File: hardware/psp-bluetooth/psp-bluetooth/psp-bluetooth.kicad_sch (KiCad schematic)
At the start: 16 parts, among them J1 Left Connector, J2 Center Connector, J3 Right Connector, J4 Analog Connector, J5 PSP Power out, J6 Power IN, J7 Serial, J8 Vin Toggle, P1 Digital, P2 Analog, P3 CONN_01X01, P4 CONN_01X01, P5 CONN_01X01, P6 CONN_01X01, U1 MCP4251-xxxx-P

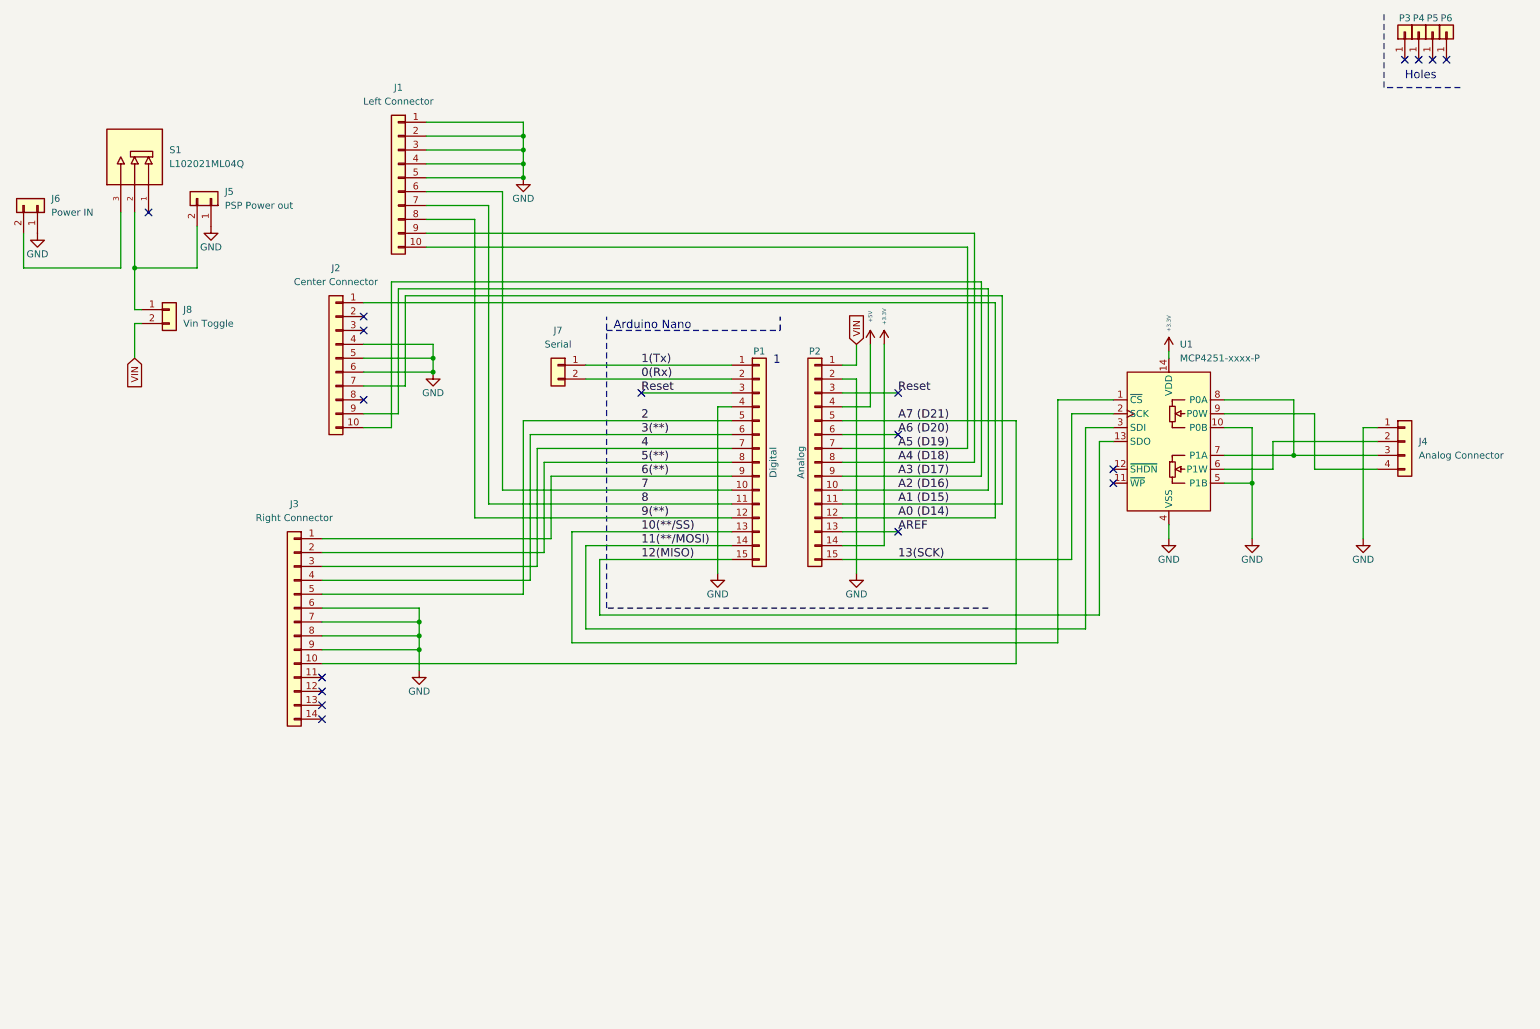
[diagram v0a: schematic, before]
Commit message: Initial work and hardware stuff
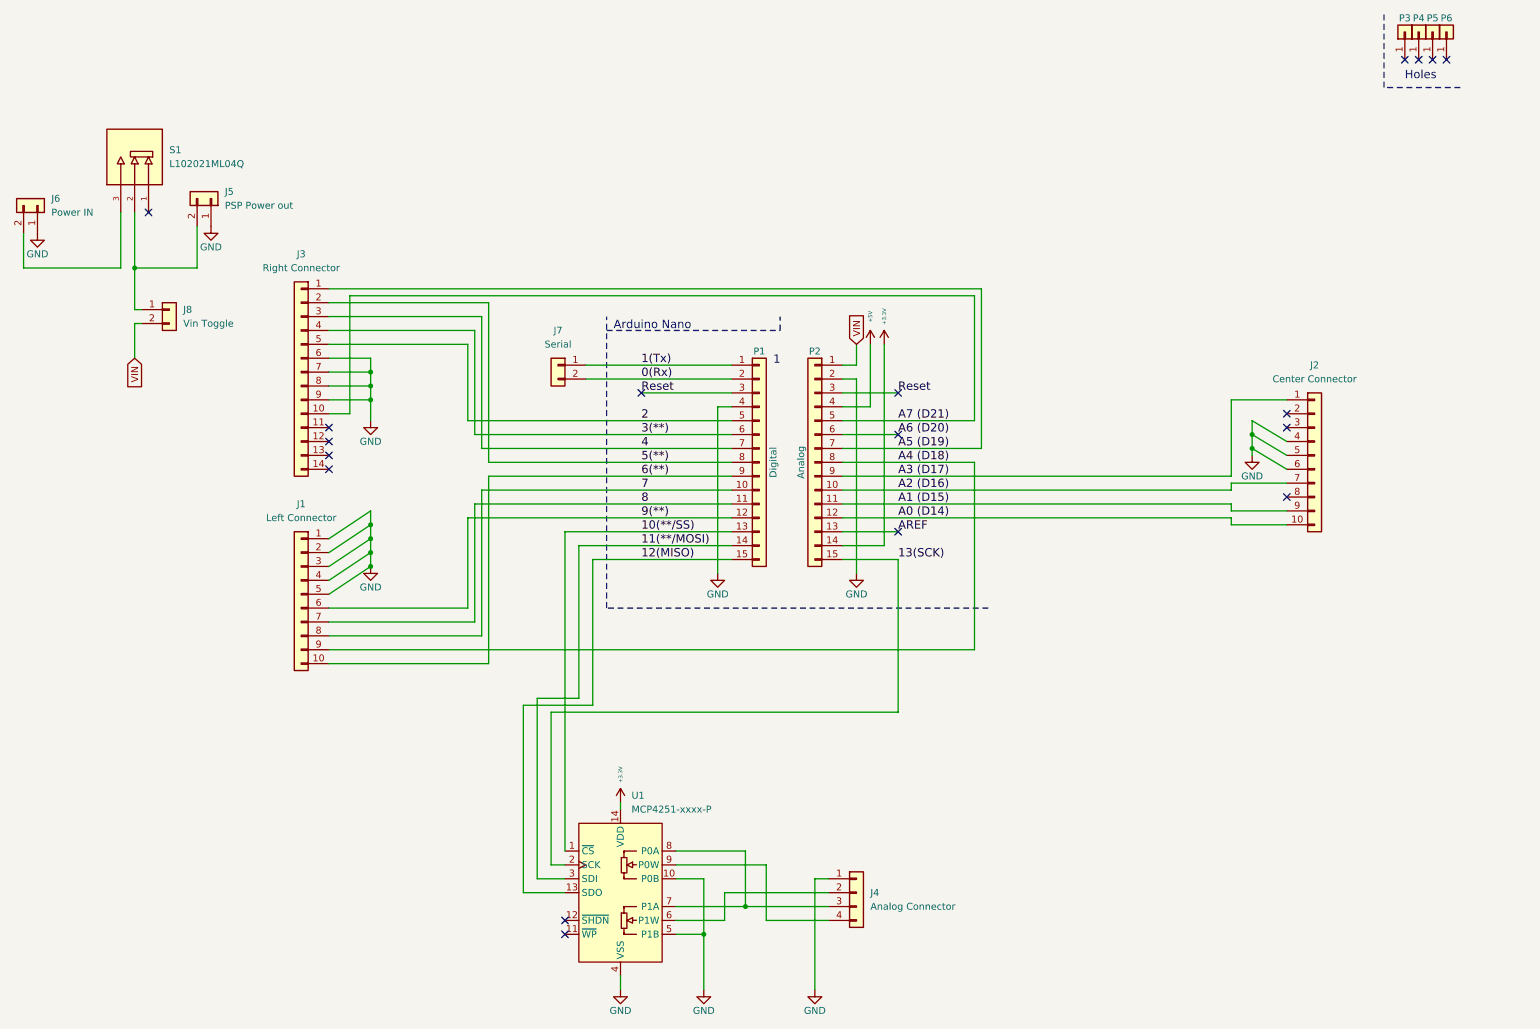
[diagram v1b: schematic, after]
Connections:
- net 6(**): now also J1.10 (Pin_10); no longer J3.1 (Pin_1)
- net 7: now also J1.8 (Pin_8); no longer J1.6 (Pin_6)
- net 9(**): now also J1.6 (Pin_6); no longer J1.8 (Pin_8)
- net A0 (D14): now also J2.10 (Pin_10); no longer J2.1 (Pin_1)
- net A1 (D15): now also J2.9 (Pin_9); no longer J2.7 (Pin_7)
- net A2 (D16): now also J2.7 (Pin_7); no longer J2.9 (Pin_9)
- net A3 (D17): now also J2.1 (Pin_1); no longer J2.10 (Pin_10)
- net A5 (D19): now also J3.1 (Pin_1); no longer J1.10 (Pin_10)
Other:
- moved on the sheet: J1, J2, J3, J4, U1
